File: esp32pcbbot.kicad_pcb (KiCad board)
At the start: 2 copper layers, 110 x 170 mm, 44 parts, among them IC1 BMI055, J1 TB002-500-02BE, J2 TB002-500-02BE, J3 TB002-500-02BE, J4 215299-4, J5 SSQ-120-01-L-D, J6 215299-4, Q1 2N7002, Q2 2N7002, Q3 Q_Photo_NPN, Q4 Q_Photo_NPN, U1 ESP32-WROOM-32E-Espressif, U2 CP2102N-A01-GQFN28, U3 L293D, U4 12BHC186P1-GR

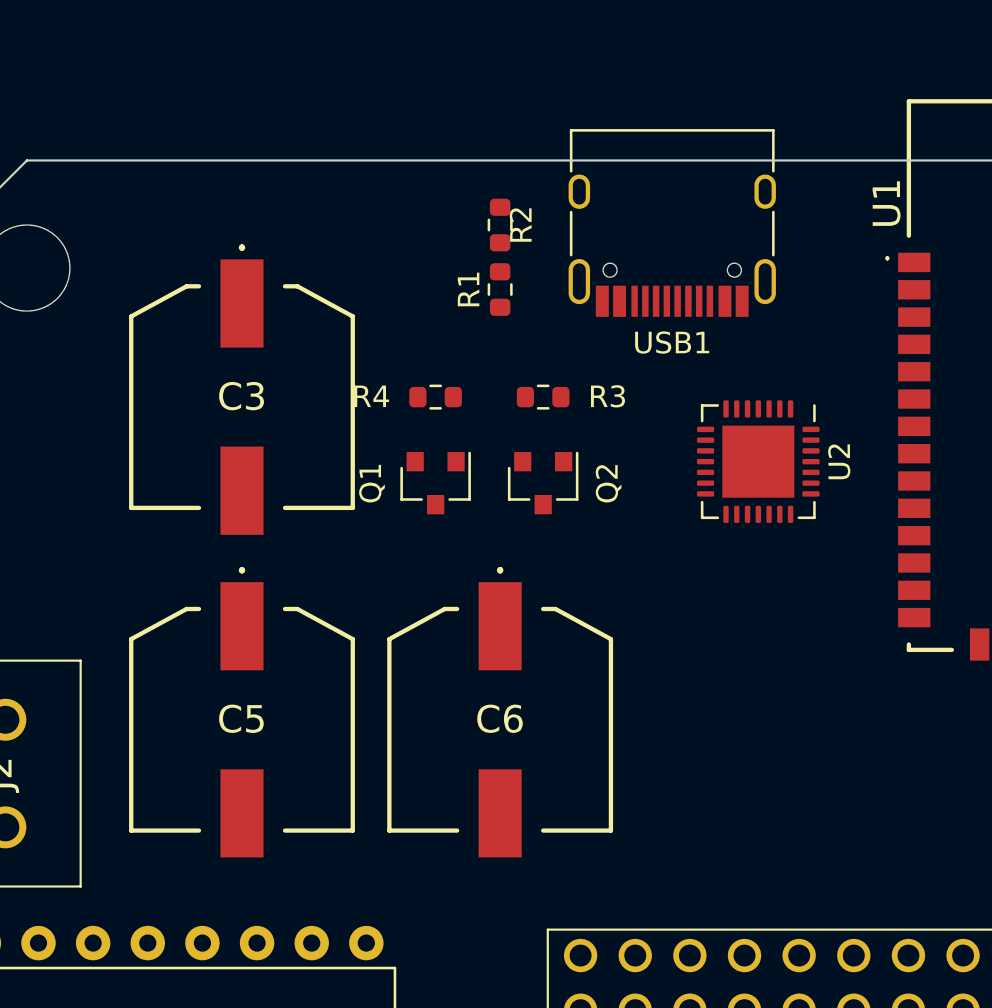
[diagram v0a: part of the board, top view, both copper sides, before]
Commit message: more autorouting shenanigins
please work i beg you pleaseworkpleaseworkpleasworkpleasework
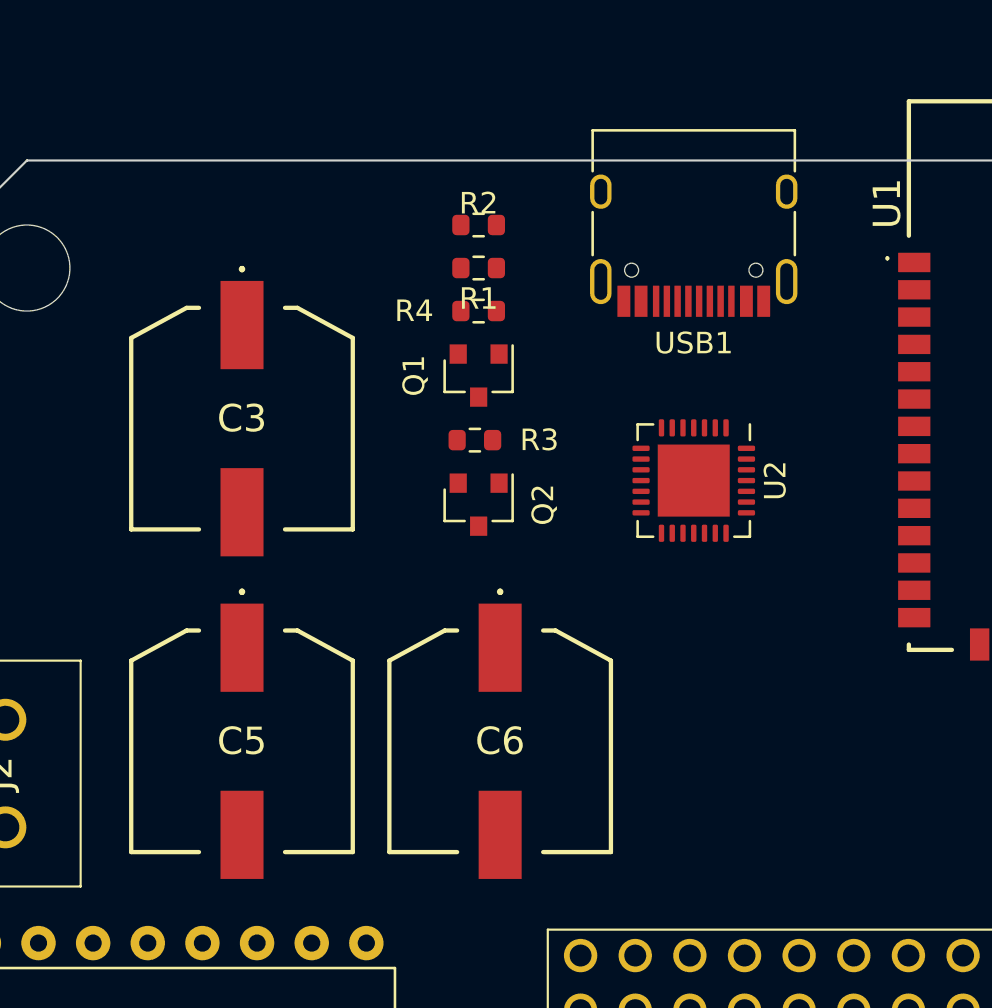
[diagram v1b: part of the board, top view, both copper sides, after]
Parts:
- moved Q1 5.39 mm to (61.0, 35.0)
- moved R4 4.47 mm to (61.0, 32.0)
- moved R3 3.75 mm to (60.8, 38.0)
- moved Q2 3.16 mm to (61.0, 41.0)
- moved U2 3.13 mm to (71.0, 39.9)
- moved R1 1.41 mm to (61.0, 30.0), turned to 180 degrees
- moved C3 1.00 mm to (50.0, 37.0)
- moved C5 1.00 mm to (50.0, 52.0)
- moved C6 1.00 mm to (62.0, 52.0)
- moved R2 1.00 mm to (61.0, 28.0), turned to 0 degrees
- moved USB1 1.00 mm to (71.0, 27.5)
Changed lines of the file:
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@@
   )
   (module SamacSys_Parts:EEEFK1V331P (layer F.Cu)
-    (at 62 51 180)
+    (at 62 52 180)
     (descr G)
     (tags "Capacitor Polarised")
@@
   )
   (module SamacSys_Parts:EEEFK1V331P (layer F.Cu)
-    (at 50 51 180)
+    (at 50 52 180)
     (descr G)
     (tags "Capacitor Polarised")
@@
   )
   (module SamacSys_Parts:EEEFK1V331P (layer F.Cu)
-    (at 50 36 180)
+    (at 50 37 180)
     (descr G)
     (tags "Capacitor Polarised")
@@
   )
   (module ESP32bot:USB_C_Receptacle_HRO_TYPE-C-31-M-12 (layer F.Cu)
-    (at 70 27.5 180)
+    (at 71 27.5 180)
     (descr "USB Type-C receptacle for USB 2.0 and PD, http://www.krhro.com/uploads/soft/180320/1-1P320120243.pdf")
     (tags "usb usb-c 2.0 pd")
@@
   )
   (module Package_DFN_QFN:QFN-28-1EP_5x5mm_P0.5mm_EP3.35x3.35mm (layer F.Cu)
-    (at 74 39 270)
+    (at 71 39.88 270)
     (descr "QFN, 28 Pin (http://ww1.microchip.com/downloads/en/PackagingSpec/00000049BQ.pdf#page=283), generated with kicad-footprint-generator ipc_noLead_generator.py")
     (tags "QFN NoLead")
@@
   )
   (module Resistor_SMD:R_0603_1608Metric (layer F.Cu)
-    (at 59 36)
+    (at 61 32)
     (descr "Resistor SMD 0603 (1608 Metric), square (rectangular) end terminal, IPC_7351 nominal, (Body size source: IPC-SM-782 page 72, https://www.pcb-3d.com/wordpress/wp-content/uploads/ipc-sm-782a_amendment_1_and_2.pdf), generated with kicad-footprint-generator")
     (tags resistor)
@@
   )
   (module Resistor_SMD:R_0603_1608Metric (layer F.Cu)
-    (at 64 36 180)
+    (at 60.825 38 180)
     (descr "Resistor SMD 0603 (1608 Metric), square (rectangular) end terminal, IPC_7351 nominal, (Body size source: IPC-SM-782 page 72, https://www.pcb-3d.com/wordpress/wp-content/uploads/ipc-sm-782a_amendment_1_and_2.pdf), generated with kicad-footprint-generator")
     (tags resistor)
@@
   )
   (module Resistor_SMD:R_0603_1608Metric (layer F.Cu)
-    (at 62 28 270)
+    (at 61 28)
     (descr "Resistor SMD 0603 (1608 Metric), square (rectangular) end terminal, IPC_7351 nominal, (Body size source: IPC-SM-782 page 72, https://www.pcb-3d.com/wordpress/wp-content/uploads/ipc-sm-782a_amendment_1_and_2.pdf), generated with kicad-footprint-generator")
     (tags resistor)
     (attr smd)
-    (fp_text reference R2 (at 0 -1 90) (layer F.SilkS)
-      (effects (font (size 1 1) (thickness 0.15)))
-    )
-    (fp_text value 5.11k (at 0 1.43 90) (layer F.Fab)
+    (fp_text reference R2 (at 0 -1) (layer F.SilkS)
+      (effects (font (size 1 1) (thickness 0.15)))
+    )
+    (fp_text value 5.11k (at 0 1.43) (layer F.Fab)
       (effects (font (size 1 1) (thickness 0.15)))
     )
@@
     (fp_line (start 1.48 -0.73) (end 1.48 0.73) (layer F.CrtYd) (width 0.05))
     (fp_line (start 1.48 0.73) (end -1.48 0.73) (layer F.CrtYd) (width 0.05))
-    (fp_text user %R (at -1 -1 90) (layer F.Fab)
+    (fp_text user %R (at -1 -1) (layer F.Fab)
       (effects (font (size 0.4 0.4) (thickness 0.06)))
     )
-    (pad 2 smd roundrect (at 0.825 0 270) (size 0.8 0.95) (layers F.Cu F.Paste F.Mask) (roundrect_rratio 0.25)
-      (net 2 GND))
-    (pad 1 smd roundrect (at -0.825 0 270) (size 0.8 0.95) (layers F.Cu F.Paste F.Mask) (roundrect_rratio 0.25)
+    (pad 2 smd roundrect (at 0.825 0) (size 0.8 0.95) (layers F.Cu F.Paste F.Mask) (roundrect_rratio 0.25)
+      (net 2 GND))
+    (pad 1 smd roundrect (at -0.825 0) (size 0.8 0.95) (layers F.Cu F.Paste F.Mask) (roundrect_rratio 0.25)
       (net 58 "Net-(R2-Pad1)"))
     (model ${KISYS3DMOD}/Resistor_SMD.3dshapes/R_0603_1608Metric.wrl
@@
   )
   (module Resistor_SMD:R_0603_1608Metric (layer F.Cu)
-    (at 62 31 90)
+    (at 61 30 180)
     (descr "Resistor SMD 0603 (1608 Metric), square (rectangular) end terminal, IPC_7351 nominal, (Body size source: IPC-SM-782 page 72, https://www.pcb-3d.com/wordpress/wp-content/uploads/ipc-sm-782a_amendment_1_and_2.pdf), generated with kicad-footprint-generator")
     (tags resistor)
     (attr smd)
-    (fp_text reference R1 (at 0 -1.43 90) (layer F.SilkS)
-      (effects (font (size 1 1) (thickness 0.15)))
-    )
-    (fp_text value 5.11k (at 0 1.43 90) (layer F.Fab)
+    (fp_text reference R1 (at 0 -1.43) (layer F.SilkS)
+      (effects (font (size 1 1) (thickness 0.15)))
+    )
+    (fp_text value 5.11k (at 0 1.43) (layer F.Fab)
       (effects (font (size 1 1) (thickness 0.15)))
     )
@@
     (fp_line (start 1.48 -0.73) (end 1.48 0.73) (layer F.CrtYd) (width 0.05))
     (fp_line (start 1.48 0.73) (end -1.48 0.73) (layer F.CrtYd) (width 0.05))
-    (fp_text user %R (at 0 0 180) (layer F.Fab)
+    (fp_text user %R (at 0 0 270) (layer F.Fab)
       (effects (font (size 0.4 0.4) (thickness 0.06)))
     )
-    (pad 2 smd roundrect (at 0.825 0 90) (size 0.8 0.95) (layers F.Cu F.Paste F.Mask) (roundrect_rratio 0.25)
-      (net 2 GND))
-    (pad 1 smd roundrect (at -0.825 0 90) (size 0.8 0.95) (layers F.Cu F.Paste F.Mask) (roundrect_rratio 0.25)
+    (pad 2 smd roundrect (at 0.825 0 180) (size 0.8 0.95) (layers F.Cu F.Paste F.Mask) (roundrect_rratio 0.25)
+      (net 2 GND))
+    (pad 1 smd roundrect (at -0.825 0 180) (size 0.8 0.95) (layers F.Cu F.Paste F.Mask) (roundrect_rratio 0.25)
       (net 57 "Net-(R1-Pad1)"))
     (model ${KISYS3DMOD}/Resistor_SMD.3dshapes/R_0603_1608Metric.wrl
@@
   )
   (module Package_TO_SOT_SMD:SOT-23 (layer F.Cu)
-    (at 64 40 270)
+    (at 61 41 270)
     (descr "SOT-23, Standard")
     (tags SOT-23)
@@
   )
   (module Package_TO_SOT_SMD:SOT-23 (layer F.Cu)
-    (at 59 40 270)
+    (at 61 35 270)
     (descr "SOT-23, Standard")
     (tags SOT-23)
